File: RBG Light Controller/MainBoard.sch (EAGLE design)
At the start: 19 parts, among them IC1 74HC595N, IC2 4584N, U1 ARDUINOR3-BPLACE

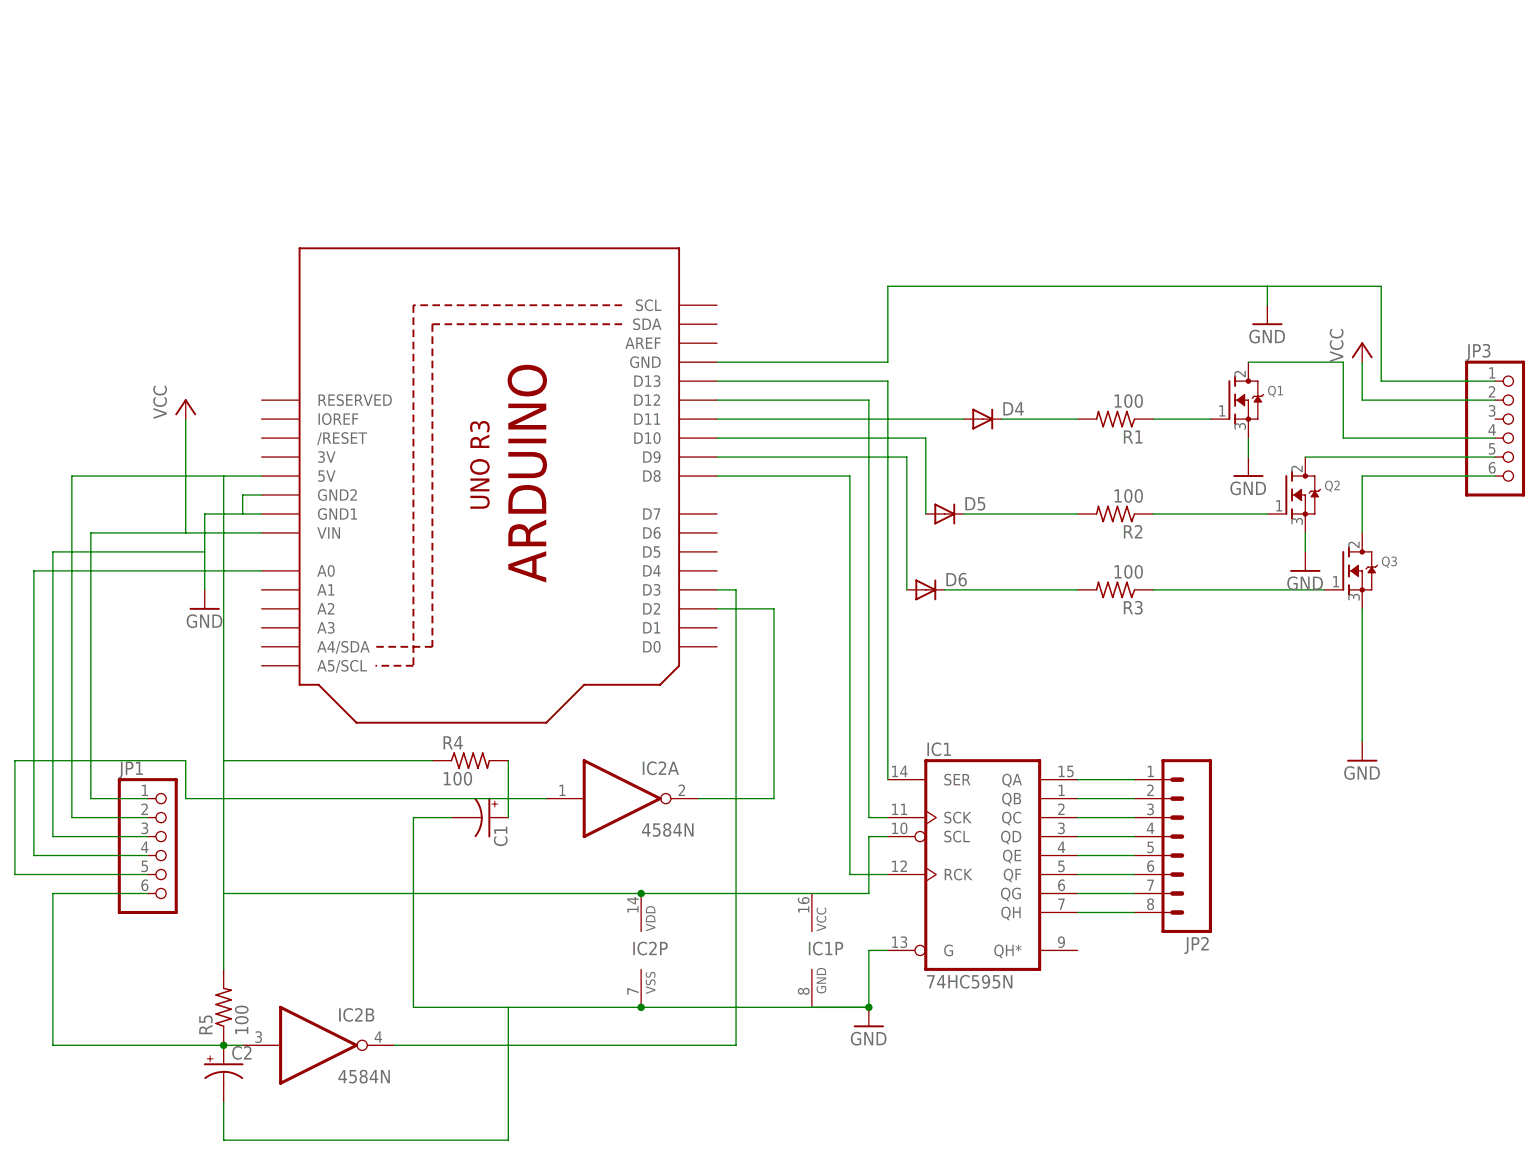
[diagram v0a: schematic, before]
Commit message: updated schematic
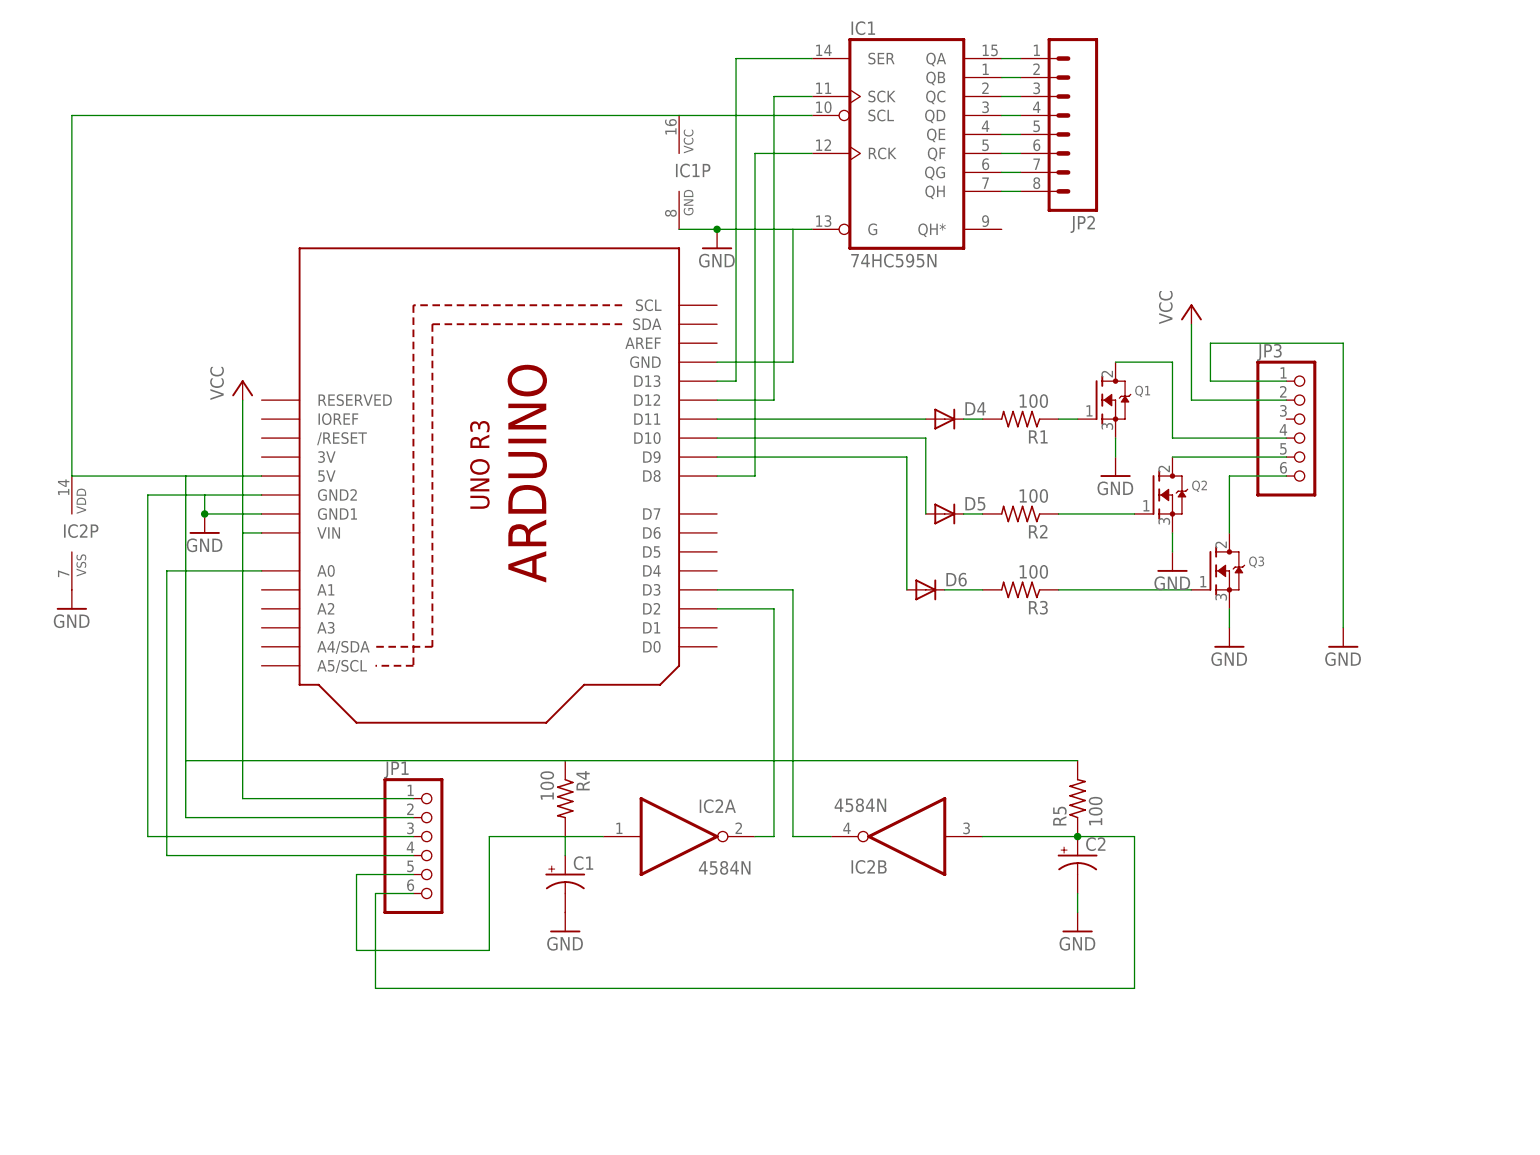
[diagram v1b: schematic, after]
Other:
- moved on the sheet: C1, C2, D4, IC1, IC1P, IC2A, IC2B, IC2P, JP1, JP2, JP3, Q1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
